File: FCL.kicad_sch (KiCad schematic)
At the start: 4 parts

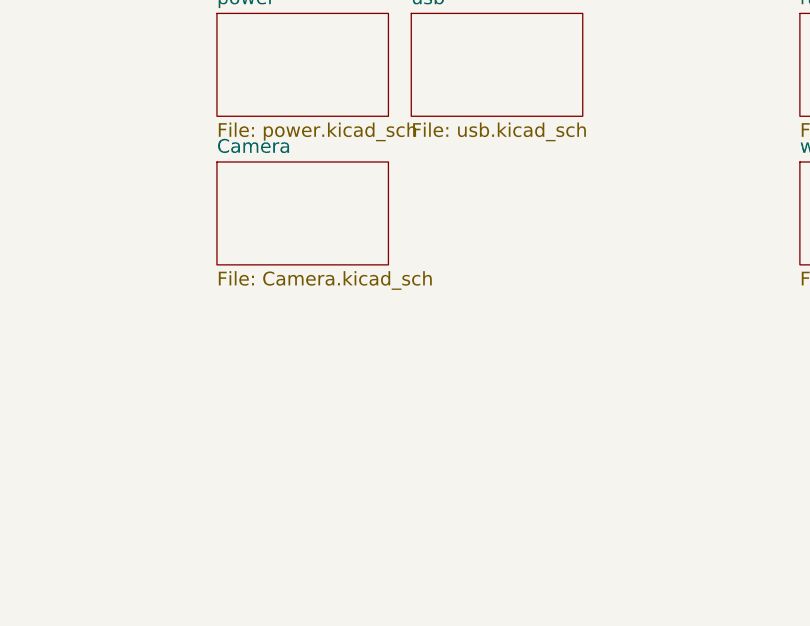
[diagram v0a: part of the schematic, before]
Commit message: AI 1st attempt at add camera.
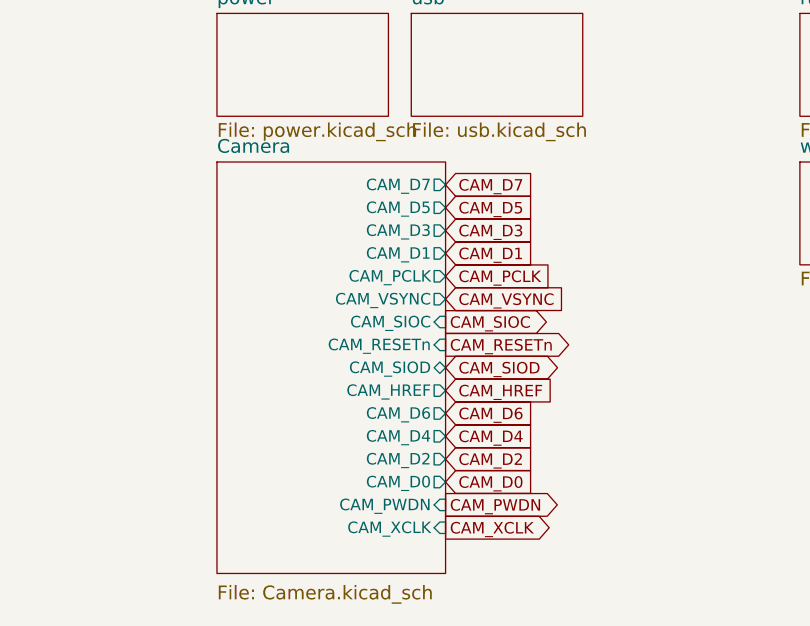
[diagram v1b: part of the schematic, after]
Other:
- sheet Camera ports: added CAM_D0, CAM_D1, CAM_D2, CAM_D3, CAM_D4, CAM_D5, CAM_D6, CAM_D7, CAM_HREF, CAM_PCLK, CAM_PWDN, CAM_RESETn, CAM_SIOC, CAM_SIOD, CAM_VSYNC, CAM_XCLK; removed none
